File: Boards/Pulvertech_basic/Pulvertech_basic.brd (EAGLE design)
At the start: 76.2 x 38.4 mm, 23 parts, among them IC1 786TV, K3 G5LE, Q2 BC548, U2 ATTINY85-20PU

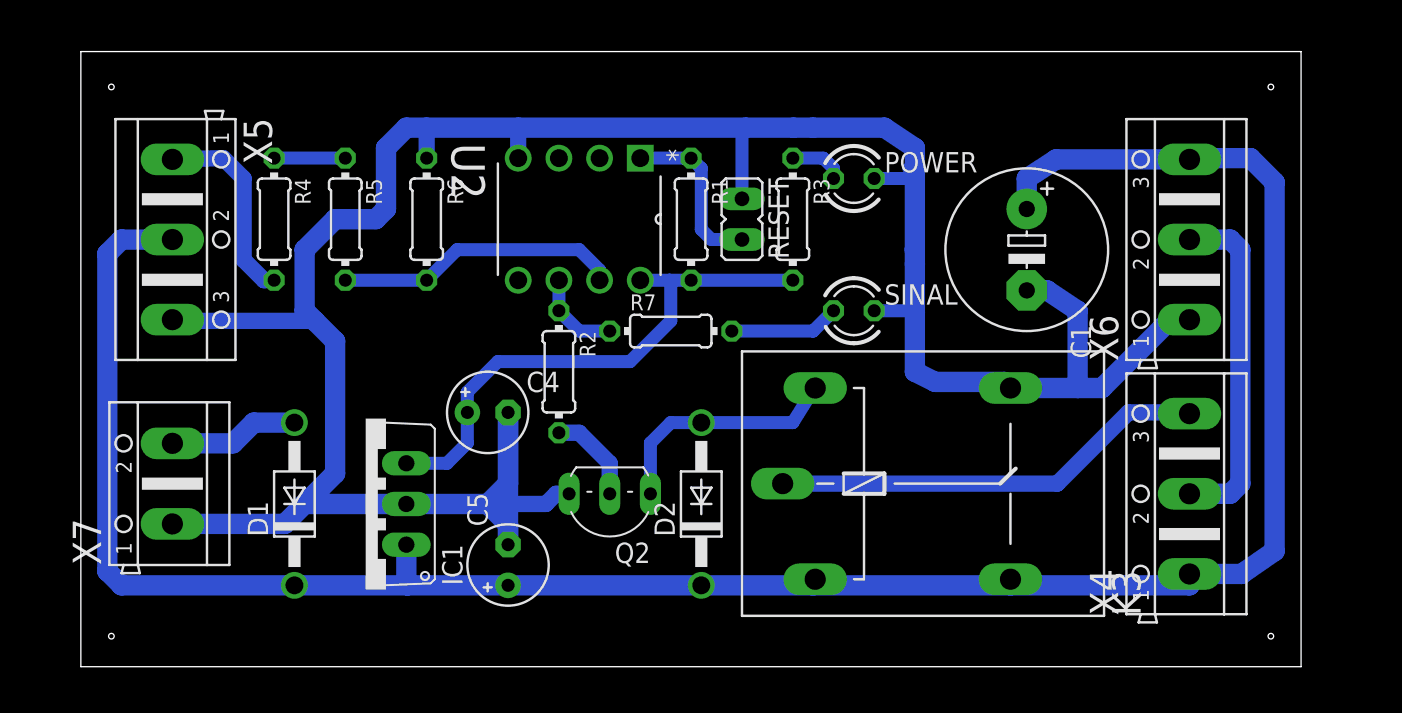
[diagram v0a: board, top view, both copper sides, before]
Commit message: update for manufactoring
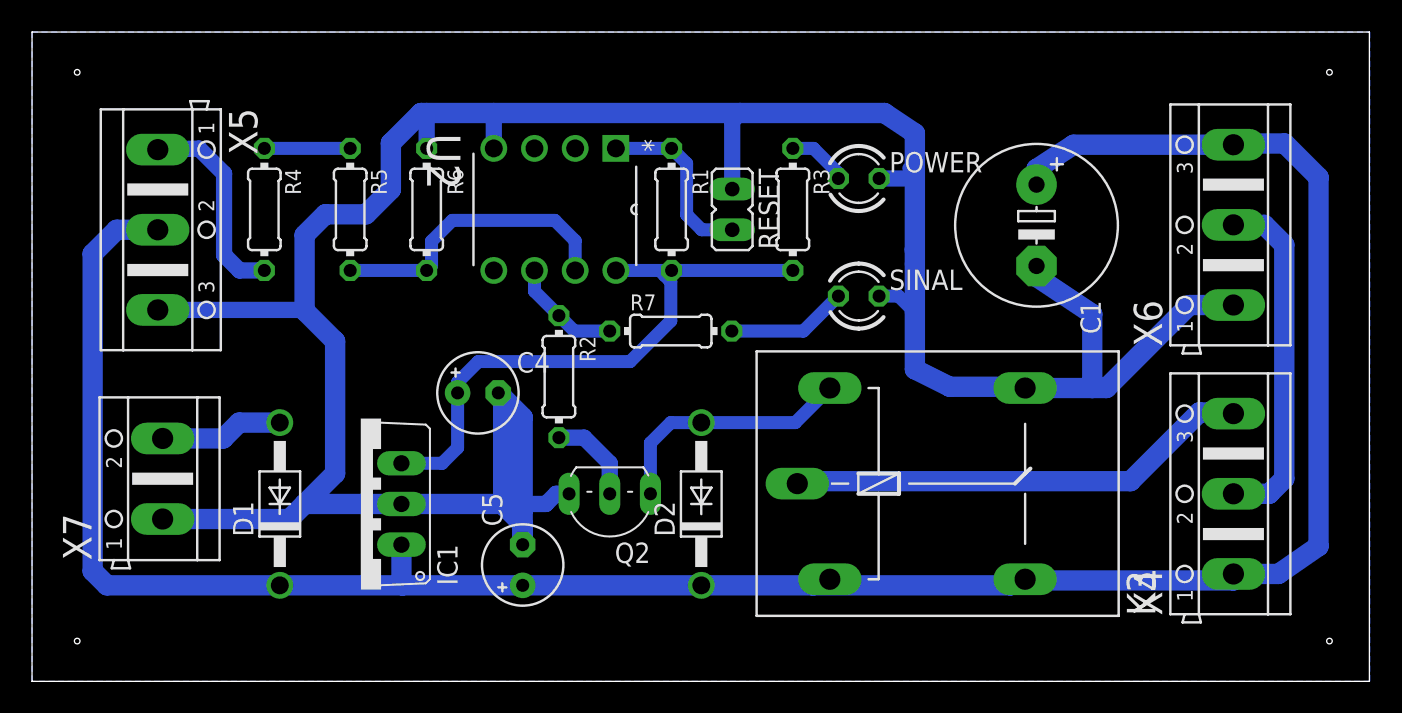
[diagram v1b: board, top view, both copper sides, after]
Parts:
- moved X6 2.89 mm to (72.0, 27.6)
- moved X4 2.74 mm to (72.0, 10.8)
- moved C1 1.64 mm to (59.7, 27.6)
- moved U2 1.64 mm to (25.8, 24.7)
- moved R1 1.36 mm to (36.9, 28.5)
- moved C4 1.36 mm to (24.8, 17.1)
- moved X5 1.10 mm to (4.80, 27.3)
- moved SINAL 0.96 mm to (48.6, 23.1)
- moved D1 0.91 mm to (12.4, 10.2)
- moved C5 0.91 mm to (27.6, 6.35)
- moved K3 0.91 mm to (54.3, 11.4)
- moved R4 0.86 mm to (11.5, 28.5)
- moved RESET 0.86 mm to (40.7, 28.5)
- moved R5 0.68 mm to (16.8, 28.5)
- moved X7 0.68 mm to (5.11, 11.7)
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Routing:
- net GND: track 171.7 -> 185.7 mm
- net VIN: track 144.8 -> 150.5 mm
- net VCC: track 34.2 -> 37.4 mm
- net AUTO_VALVE: track 27.3 -> 29.1 mm
- net VALVE_SIGN: track 5.61 -> 7.03 mm
- net N$31: track 4.45 -> 5.36 mm
- net SENSOR_IND: track 17.8 -> 18.6 mm
- net N$6: track 6.88 -> 7.56 mm
- net N$13: track 15.3 -> 15.9 mm
- net N$1: track 10.7 -> 11.2 mm
- added copper zone on layer 16, net N$7
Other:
- board size 76.2 x 38.4 mm -> 83.5 x 40.5 mm
- board text added: "Aberto"
- board text added: "Auto"
- board text added: "Bateria"
- board text added: "Chave"
- board text added: "Com"
- board text added: "Sensor"
- board text added: "Valvula"
- board text removed: "2018"
- board text removed: "BATERIA"
- board text removed: "CHAVE SELETORA"
- board text removed: "FREE BIRD"
- board text removed: "POWER"
- board text removed: "PULVERTECH LITE"
- board text removed: "SENSOR"
- board text removed: "SINAL"
- board text removed: "VALVULA"
